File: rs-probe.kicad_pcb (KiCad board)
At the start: 4 copper layers, 40 x 14 mm, 108 parts, among them J1 USB_C_Receptacle_USB2.0, J10 Conn_01x01, J11 Conn_01x01, J2 Castellated Vias, J3 Castellated Vias, J4 Castellated Vias, J5 tag-connect-swd, J6 Conn_01x01, J7 Conn_01x01, J8 Conn_01x01, J9 Conn_01x01, Q1 NTZD3155C or CMLDM3757-TR-PBF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, SW1 SW_Push, T1 Tab, T2 Tab, U1 74LVC1T45GM,115, U10 74LVC1T45GM,115, U11 74LVC1T45GM,115, U12 NCP133AMXADJTCG, U13 NCP133AMXADJTCG, U14 NCP133AMXADJTCG, U2 74LVC1T45GM,115, U3 W25Q8, U4 NUF8401MNT4G, U5 CortexDebug, U6 RP2040, U7 NUF2042XV6T1G, U8 74LVC1T45GM,115, U9 74LVC1T45GM,115, X1 12 MHz

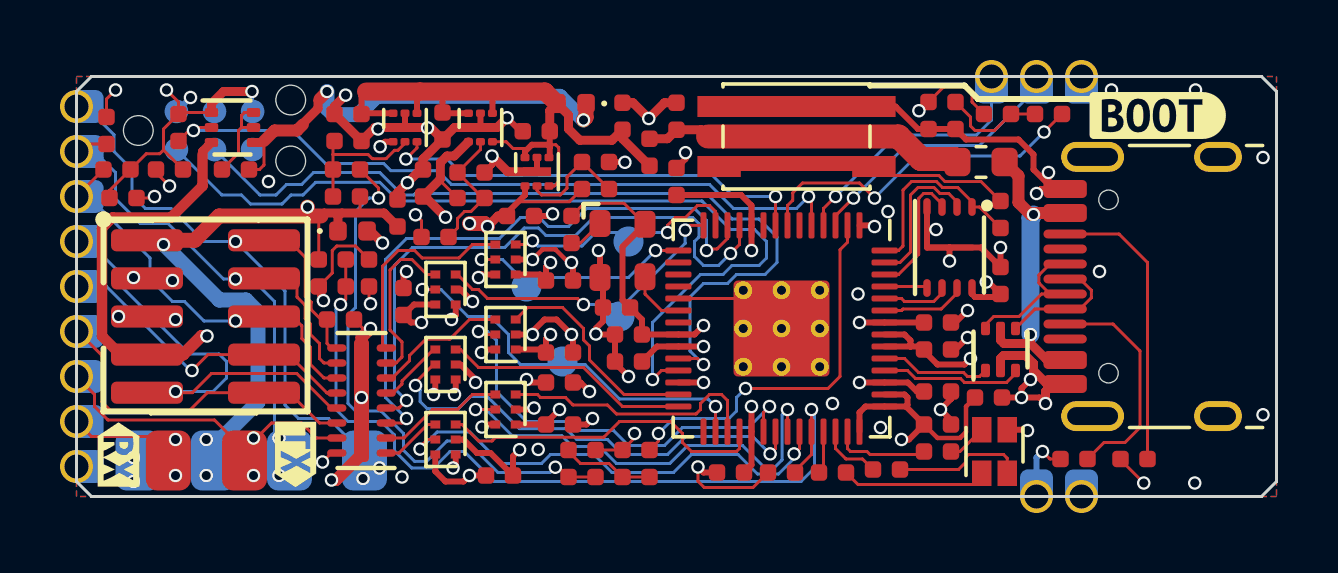
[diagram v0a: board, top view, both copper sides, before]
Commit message: Run CI for older ref
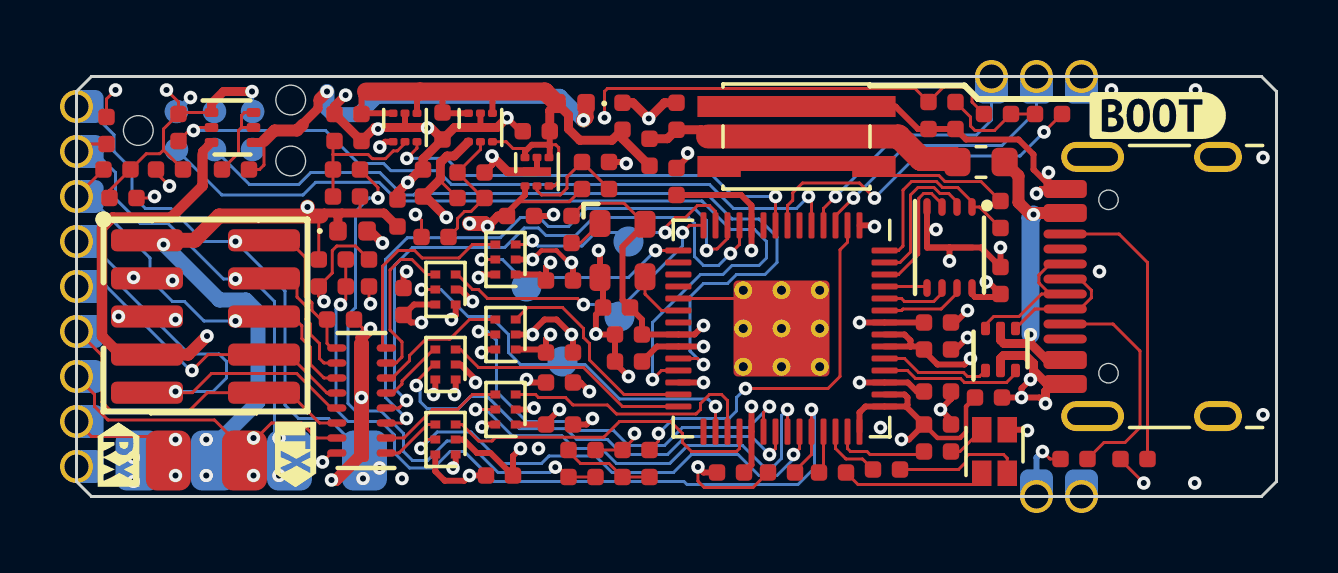
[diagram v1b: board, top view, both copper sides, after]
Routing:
- net /VS2_T: track 22.7 -> 23.4 mm
- net GND: track 99.8 -> 100.0 mm, vias 63 -> 59
- removed copper zone on B.Cu, net GND
- removed copper zone on F.Cu, net GND
